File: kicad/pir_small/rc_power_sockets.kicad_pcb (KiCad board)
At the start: 2 copper layers, 25 x 25 mm, 27 parts, among them IC1 ATTINY85, J1 PIR, J2 433MHZ, P1 ICSP, P2 ALT_PWR, P3 CONN_01X01, P4 CONN_01X01, Q1 NMOS, Q2 PMOS, SW1 SWITCH_INV, U1 MCP1755ST-3302E/DB

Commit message: Power pins
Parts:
- P2: footprint Socket_Strips:Socket_Strip_Straight_1x02 -> Pin_Headers:Pin_Header_Straight_1x02
- turned P2 to 90 degrees
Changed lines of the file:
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@@
     (links 49)
     (no_connects 0)
-    (area 147.382999 63.582999 172.533001 88.733001)
+    (area 144.000667 61.624 175.915334 93.082)
     (thickness 1.6)
-    (drawings 35)
+    (drawings 33)
     (tracks 197)
     (zones 0)
@@
   (page A4)
   (layers
-    (0 F.Cu signal hide)
-    (31 B.Cu signal hide)
+    (0 F.Cu signal)
+    (31 B.Cu signal)
     (32 B.Adhes user)
     (33 F.Adhes user)
@@
     (35 F.Paste user)
     (36 B.SilkS user)
-    (37 F.SilkS user hide)
+    (37 F.SilkS user)
     (38 B.Mask user)
     (39 F.Mask user)
@@
     )
   )
-  (module Socket_Strips:Socket_Strip_Straight_1x02 (layer F.Cu)
-    (at 156.529 86.953)
-    (descr "Through hole socket strip")
-    (tags "socket strip")
-    (fp_text reference P2 (at 0 -5.1) (layer F.SilkS) hide
-      (effects (font (size 1 1) (thickness 0.15)))
-    )
-    (fp_text value ALT_PWR (at 0 -3.1) (layer F.Fab) hide
-      (effects (font (size 1 1) (thickness 0.15)))
-    )
-    (fp_line (start -1.55 1.55) (end 0 1.55) (layer F.SilkS) (width 0.15))
-    (fp_line (start 3.81 1.27) (end 1.27 1.27) (layer F.SilkS) (width 0.15))
-    (fp_line (start -1.75 -1.75) (end -1.75 1.75) (layer F.CrtYd) (width 0.05))
-    (fp_line (start 4.3 -1.75) (end 4.3 1.75) (layer F.CrtYd) (width 0.05))
-    (fp_line (start -1.75 -1.75) (end 4.3 -1.75) (layer F.CrtYd) (width 0.05))
-    (fp_line (start -1.75 1.75) (end 4.3 1.75) (layer F.CrtYd) (width 0.05))
-    (fp_line (start 1.27 1.27) (end 1.27 -1.27) (layer F.SilkS) (width 0.15))
-    (fp_line (start 0 -1.55) (end -1.55 -1.55) (layer F.SilkS) (width 0.15))
-    (fp_line (start -1.55 -1.55) (end -1.55 1.55) (layer F.SilkS) (width 0.15))
-    (fp_line (start 1.27 -1.27) (end 3.81 -1.27) (layer F.SilkS) (width 0.15))
-    (fp_line (start 3.81 -1.27) (end 3.81 1.27) (layer F.SilkS) (width 0.15))
-    (pad 1 thru_hole rect (at 0 0) (size 2.032 2.032) (drill 1.016) (layers *.Cu *.Mask F.SilkS)
-      (net 1 GND))
-    (pad 2 thru_hole oval (at 2.54 0) (size 2.032 2.032) (drill 1.016) (layers *.Cu *.Mask F.SilkS)
-      (net 16 /VCC))
-    (model Socket_Strips.3dshapes/Socket_Strip_Straight_1x02.wrl
-      (at (xyz 0.05 0 0))
-      (scale (xyz 1 1 1))
-      (rotate (xyz 0 0 180))
-    )
-  )
   (module Pin_Headers:Pin_Header_Straight_1x01 (layer F.Cu)
     (at 149.163 70.443)
@@
     )
   )
+  (module Pin_Headers:Pin_Header_Straight_1x02 (layer F.Cu)
+    (at 156.529 86.953 90)
+    (descr "Through hole pin header")
+    (tags "pin header")
+    (fp_text reference P2 (at 0 -5.1 90) (layer F.SilkS) hide
+      (effects (font (size 1 1) (thickness 0.15)))
+    )
+    (fp_text value ALT_PWR (at 0 -3.1 90) (layer F.Fab) hide
+      (effects (font (size 1 1) (thickness 0.15)))
+    )
+    (fp_line (start 1.27 1.27) (end 1.27 3.81) (layer F.SilkS) (width 0.15))
+    (fp_line (start 1.55 -1.55) (end 1.55 0) (layer F.SilkS) (width 0.15))
+    (fp_line (start -1.75 -1.75) (end -1.75 4.3) (layer F.CrtYd) (width 0.05))
+    (fp_line (start 1.75 -1.75) (end 1.75 4.3) (layer F.CrtYd) (width 0.05))
+    (fp_line (start -1.75 -1.75) (end 1.75 -1.75) (layer F.CrtYd) (width 0.05))
+    (fp_line (start -1.75 4.3) (end 1.75 4.3) (layer F.CrtYd) (width 0.05))
+    (fp_line (start 1.27 1.27) (end -1.27 1.27) (layer F.SilkS) (width 0.15))
+    (fp_line (start -1.55 0) (end -1.55 -1.55) (layer F.SilkS) (width 0.15))
+    (fp_line (start -1.55 -1.55) (end 1.55 -1.55) (layer F.SilkS) (width 0.15))
+    (fp_line (start -1.27 1.27) (end -1.27 3.81) (layer F.SilkS) (width 0.15))
+    (fp_line (start -1.27 3.81) (end 1.27 3.81) (layer F.SilkS) (width 0.15))
+    (pad 1 thru_hole rect (at 0 0 90) (size 2.032 2.032) (drill 1.016) (layers *.Cu *.Mask F.SilkS)
+      (net 1 GND))
+    (pad 2 thru_hole oval (at 0 2.54 90) (size 2.032 2.032) (drill 1.016) (layers *.Cu *.Mask F.SilkS)
+      (net 16 /VCC))
+    (model Pin_Headers.3dshapes/Pin_Header_Straight_1x02.wrl
+      (at (xyz 0 -0.05 0))
+      (scale (xyz 1 1 1))
+      (rotate (xyz 0 0 90))
+    )
+  )
   (gr_text A0 (at 151.449 70.316) (layer B.SilkS)
     (effects (font (size 1.016 1.016) (thickness 0.1524)) (justify mirror))
@@
     (effects (font (size 1.016 1.016) (thickness 0.1524)))
   )
-  (gr_line (start 142.458 76.158) (end 174.958 76.158) (angle 90) (layer Cmts.User) (width 0.2))
-  (gr_line (start 159.958 56.158) (end 159.958 91.158) (angle 90) (layer Cmts.User) (width 0.2))
   (gr_line (start 147.458 88.658) (end 147.458 63.658) (angle 90) (layer Edge.Cuts) (width 0.15))
   (gr_line (start 172.458 88.658) (end 147.458 88.658) (angle 90) (layer Edge.Cuts) (width 0.15))

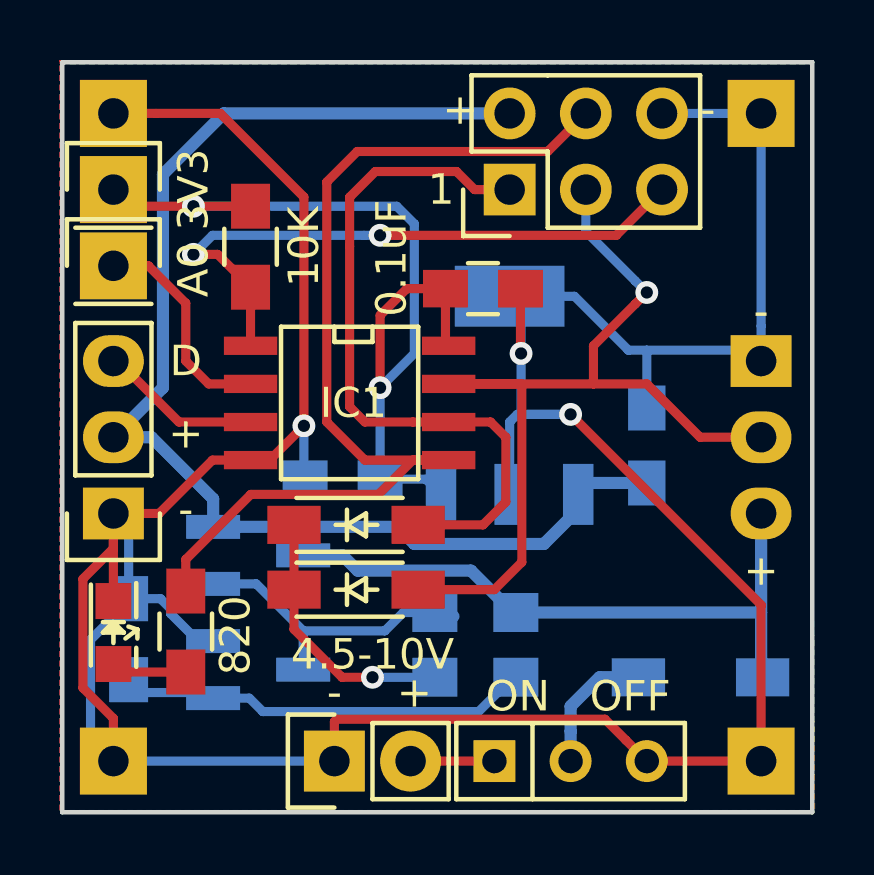
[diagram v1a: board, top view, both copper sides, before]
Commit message: Logo
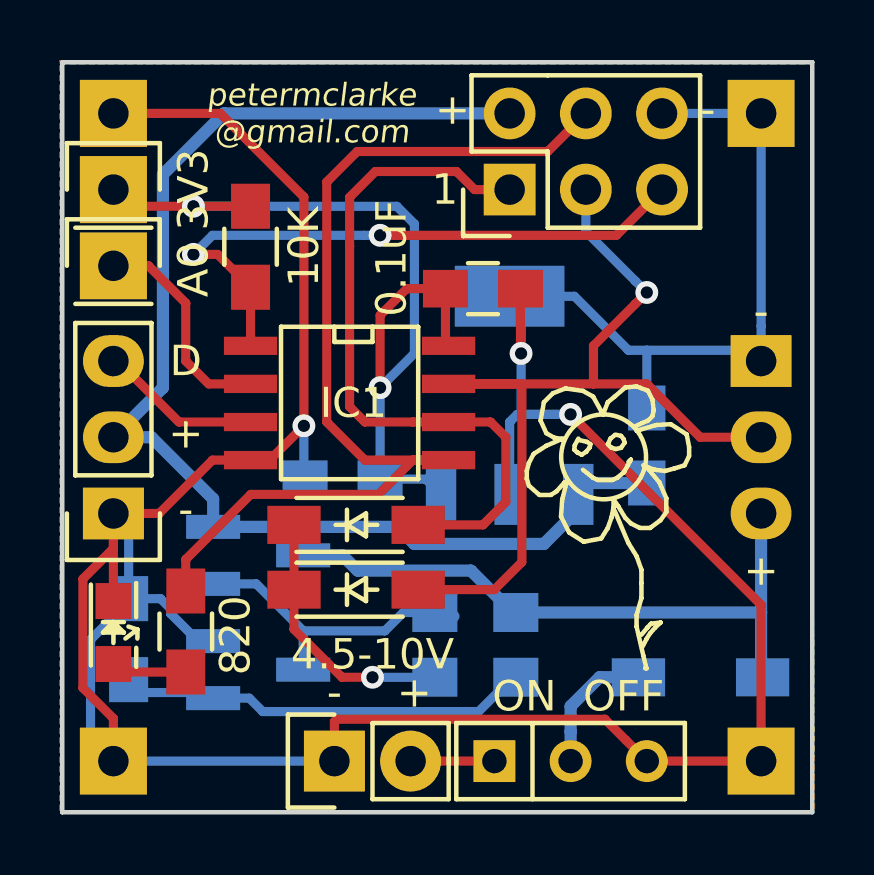
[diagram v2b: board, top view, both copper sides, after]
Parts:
- added REF**: TheApiLogo, theapi_footprints:TheApiLogoSmall, F.Cu at (165.7, 73.9)
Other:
- board text added: "petermclarke @gmail.com"
